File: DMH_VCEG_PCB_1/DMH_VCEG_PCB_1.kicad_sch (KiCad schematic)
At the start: 0 parts

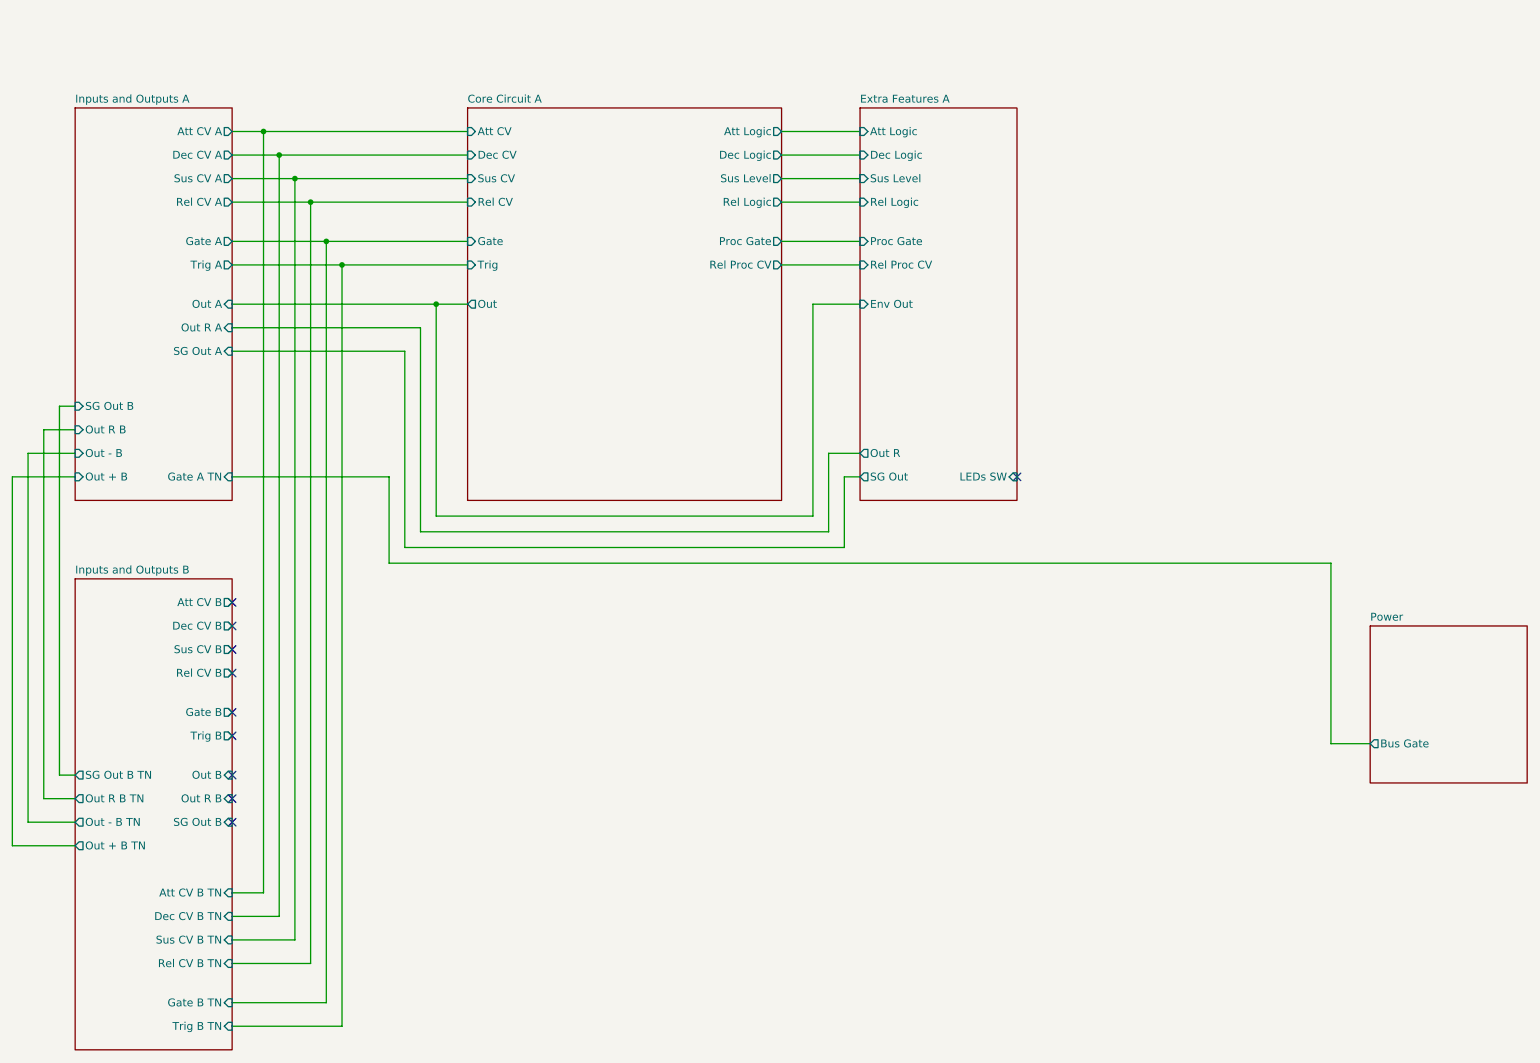
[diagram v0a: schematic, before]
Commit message: Placed Circuit B pages
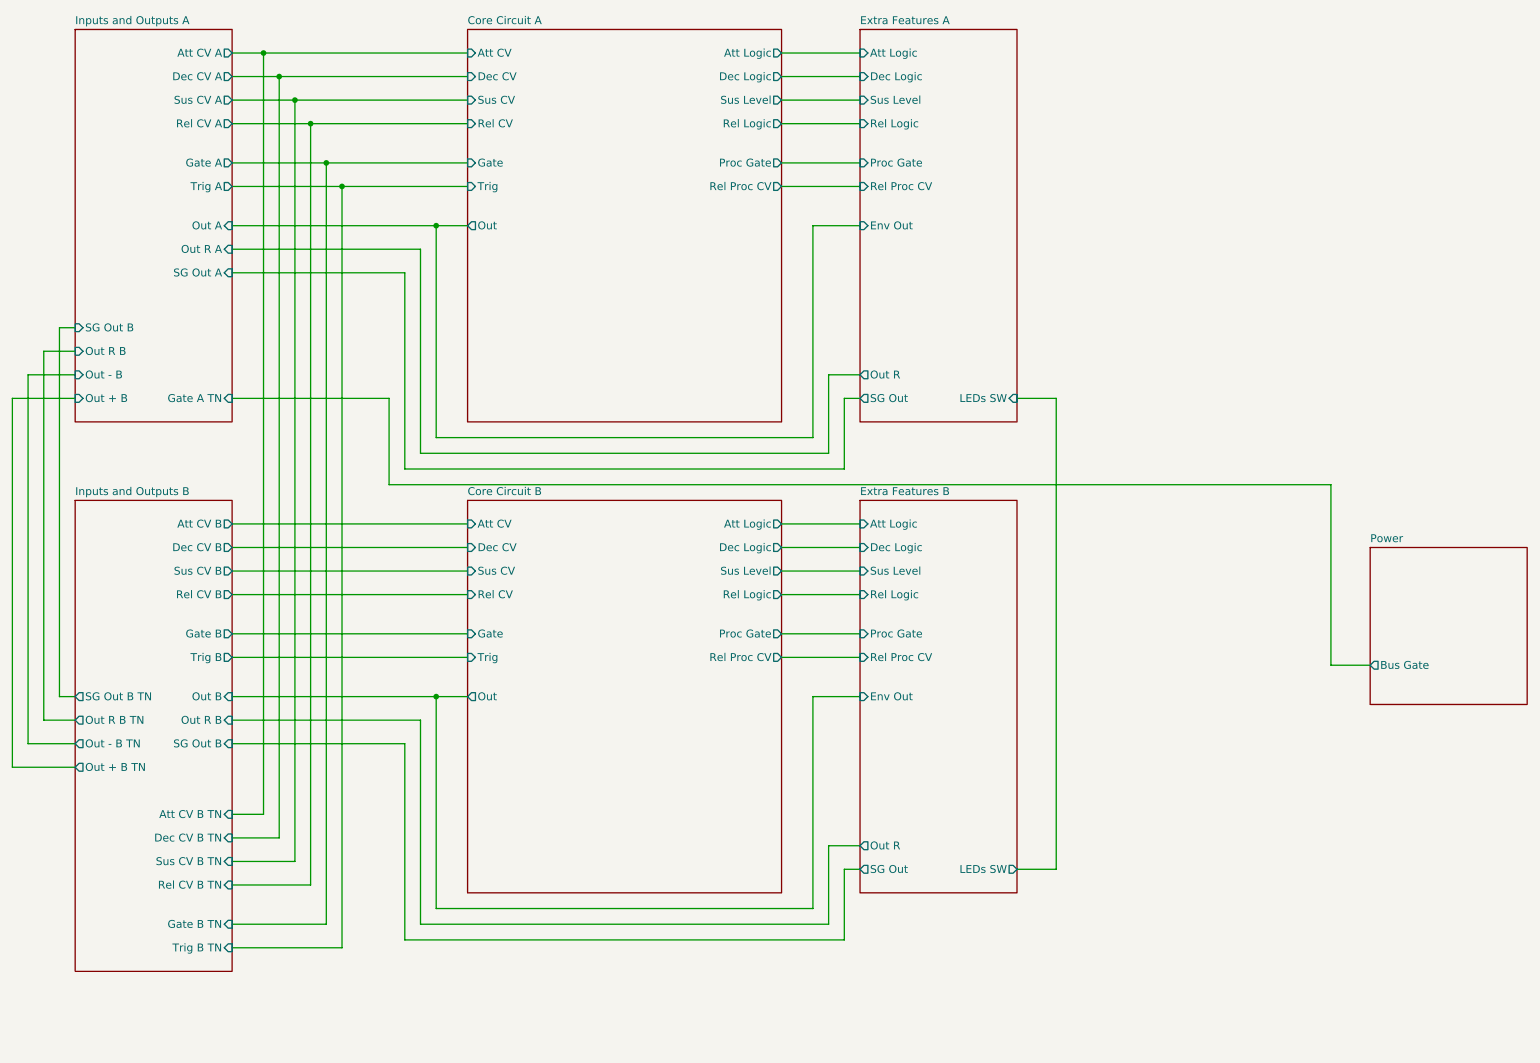
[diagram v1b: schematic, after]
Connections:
- no-connect marks 10 -> 0
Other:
- added sheet Core Circuit B (Core_Circuit_B.kicad_sch)
- added sheet Extra Features B (Extra_Features_B.kicad_sch)
